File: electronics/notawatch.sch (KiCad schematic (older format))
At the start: 25 parts, among them SW1 SW_Push, SW2 SW_Push, SW3 SW_Push, SW4 SW_Push, U1 ATtiny84A-SSU, U2 DS1307Z+, U3 HT16K33-24, U4 KWM-20882AVB, U5 SPX3819M5-L-5-0, Y1 32768Hz

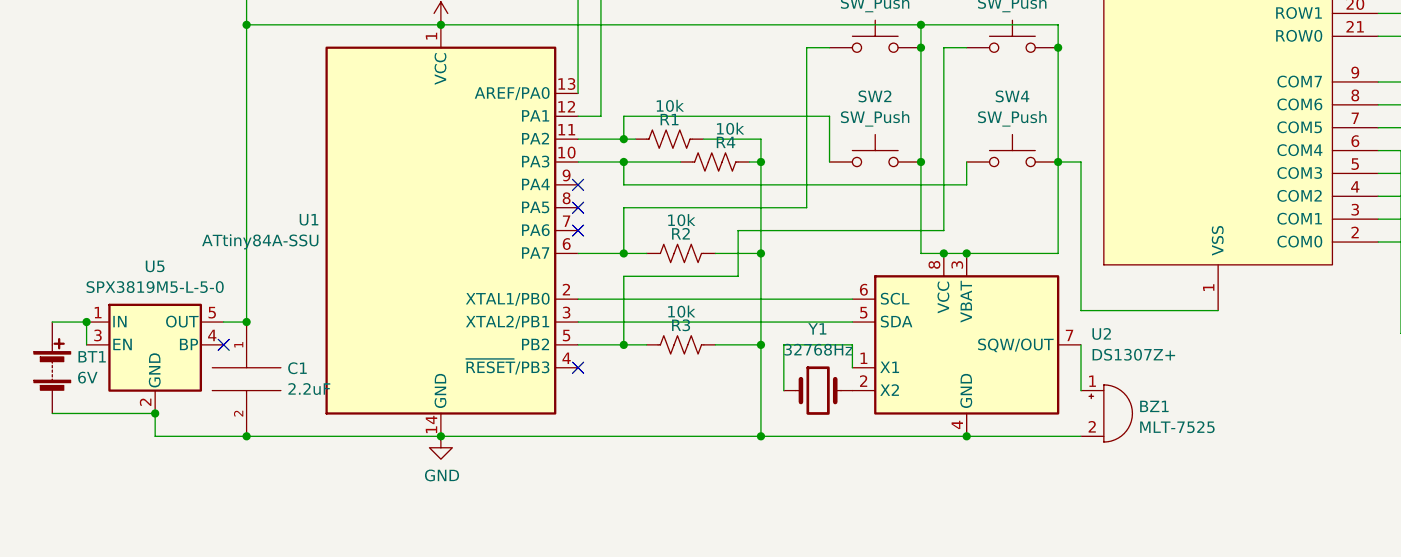
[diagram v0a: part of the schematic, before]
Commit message: Wrote code
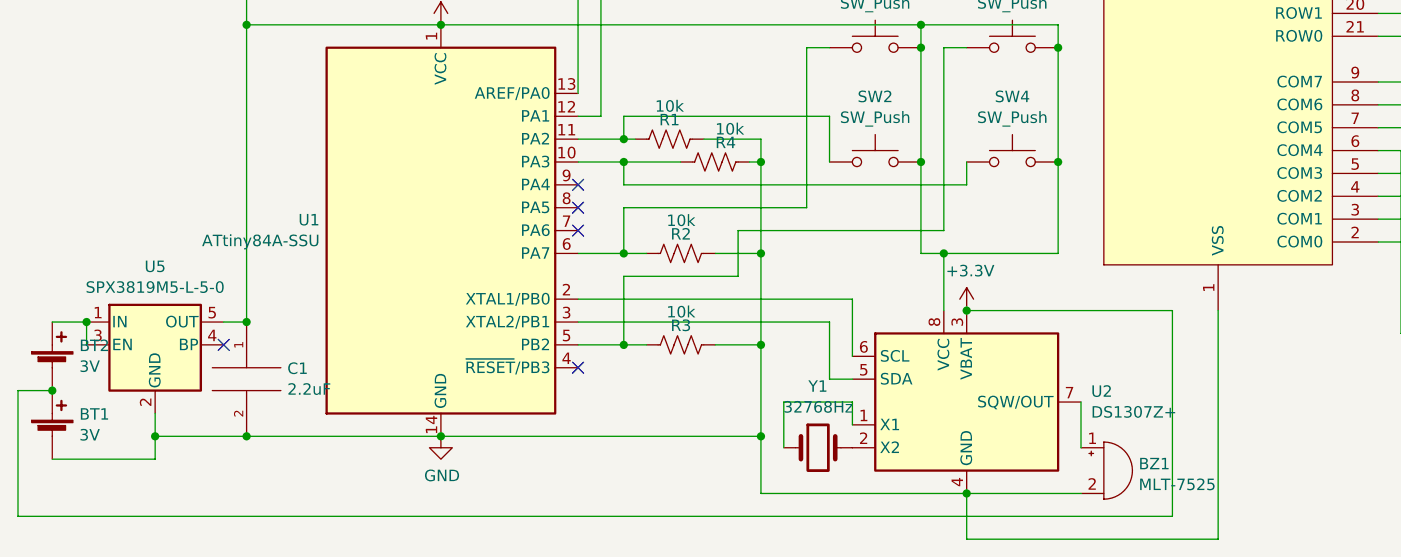
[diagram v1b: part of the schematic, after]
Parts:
- removed BT1: 6V, Connector_PinHeader_2.54mm:PinHeader_1x02_P2.54mm_Horizontal, symbol Device:Battery
- added BT1, BT2: 3V, symbol Device:Battery_Cell
- R1, R10, R11, R12, R2, R3, R4, R5, R6, R7, R8, R9: footprint Resistor_SMD:R_0201_0603Metric -> Resistor_SMD:R_0603_1608Metric
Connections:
- net labels added: +3.3V
- wire segments 136 -> 146
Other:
- moved on the sheet: BZ1, U2, Y1

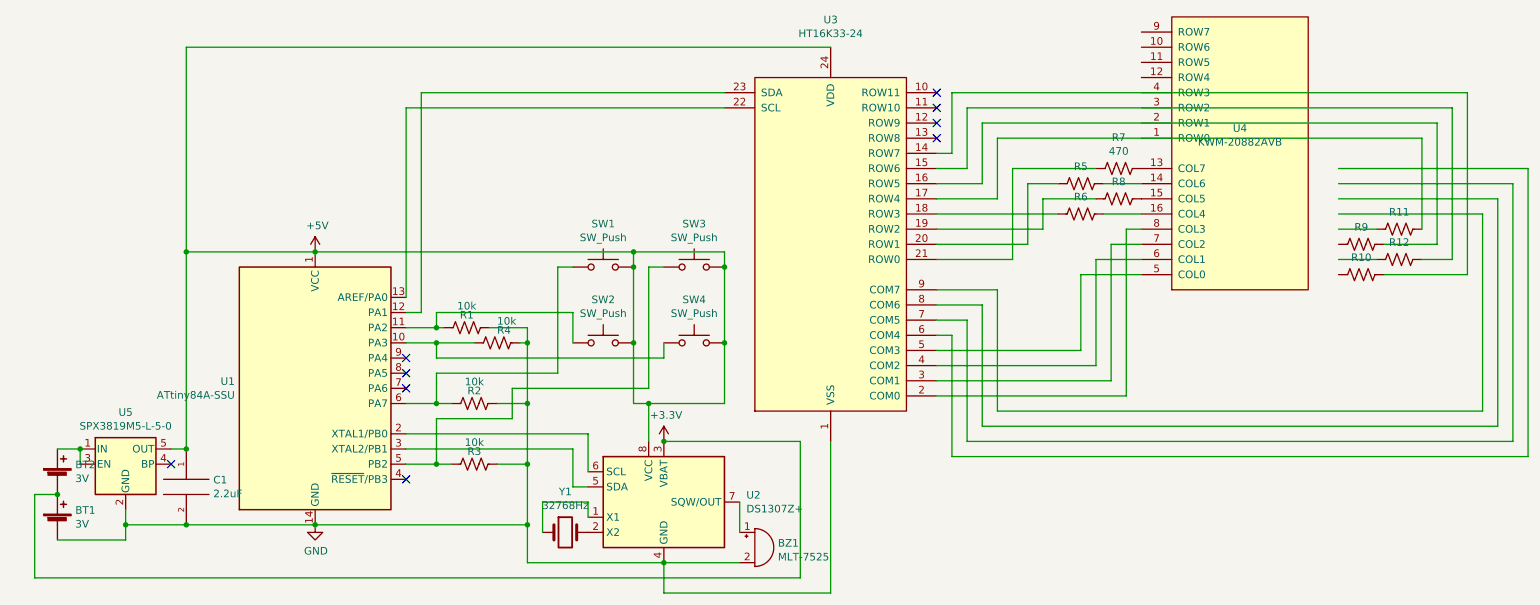
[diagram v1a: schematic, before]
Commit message: Trust me, I'm usually more dilligent about documenting git changes
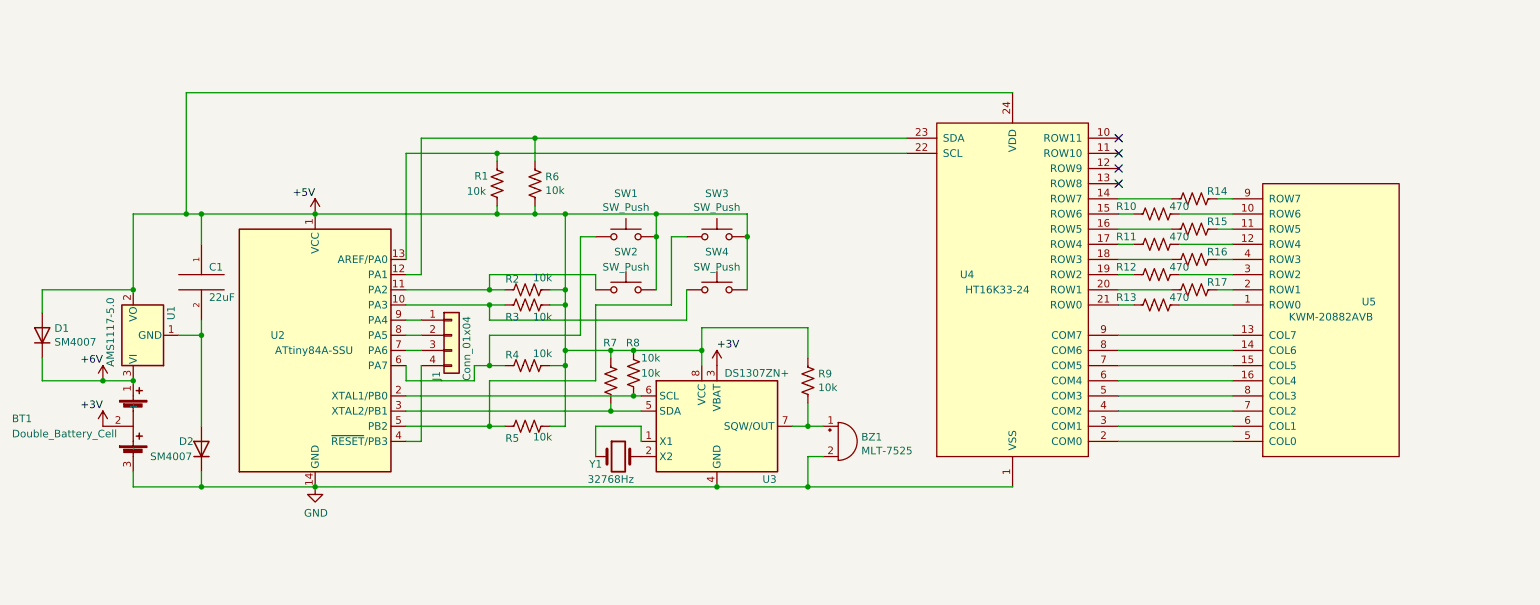
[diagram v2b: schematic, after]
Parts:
- removed BT1, BT2: 3V, symbol Device:Battery_Cell
- removed U2: DS1307Z+, Package_SO:SOIC-8_3.9x4.9mm_P1.27mm, symbol Timer_RTC:DS1307Z+
- removed U5: SPX3819M5-L-5-0, Package_TO_SOT_SMD:SOT-23-5, symbol Regulator_Linear:SPX3819M5-L-5-0
- added BT1: Double_Battery_Cell, Connector_PinHeader_2.54mm:PinHeader_1x03_P2.54mm_Vertical, symbol LED_matrix:Double_Battery_Cell
- added D1, D2: SM4007, Diode_SMD:D_MELF, symbol Diode:SM4007
- added J1: Conn_01x04, Connector_PinHeader_2.54mm:PinHeader_1x04_P2.54mm_Vertical, symbol Connector_Generic:Conn_01x04
- added R1, R6, R7, R8, R9: 10k, Resistor_SMD:R_0603_1608Metric, symbol Device:R_US
- added U1: AMS1117-5.0, Package_TO_SOT_SMD:SOT-223-3_TabPin2, symbol Regulator_Linear:AMS1117-5.0
- added U3: DS1307ZN+, Package_SO:SOIC-8_3.9x4.9mm_P1.27mm, symbol Timer_RTC:DS1307ZN+
- C1: value 2.2uF -> 22uF
- renumbered R5 to R10, R6 to R11, R9 to R12, R10 to R13, R7 to R14, R8 to R15, R11 to R16, R12 to R17, R1 to R2, R4 to R3, R2 to R4, R3 to R5, U1 to U2, U3 to U4, U4 to U5
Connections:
- net labels added: +3V, +6V, +BATT
- wire segments 146 -> 128
- no-connect marks 9 -> 4
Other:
- moved on the sheet: BZ1, C1, R10, R11, R12, R13, R14, R15, R16, R17, R2, R3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
